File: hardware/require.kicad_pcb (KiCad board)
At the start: 6 copper layers, 68 x 26 mm, 180 parts, among them J800 Molex 47346-0001, Q110 LN235N3T5G, Q840 LMBT3904DW1T1G, SW850 SW_SKSC_4PIN, U100 RK3308, U200 SY8089AAC, U220 PAM2305CGFADJ, U230 PAM2305CGFADJ, U250 PAM2305CGFADJ, U260 NCP707_XDFN4, U300 DDR3_FBGA96, U400 EMMC_BGA_153, U500 ap6255, U830 ATECC608A-MAHDA, Y100 24MHz,12pF,10ppm, Y520 37.4MHz,12pF,10ppm

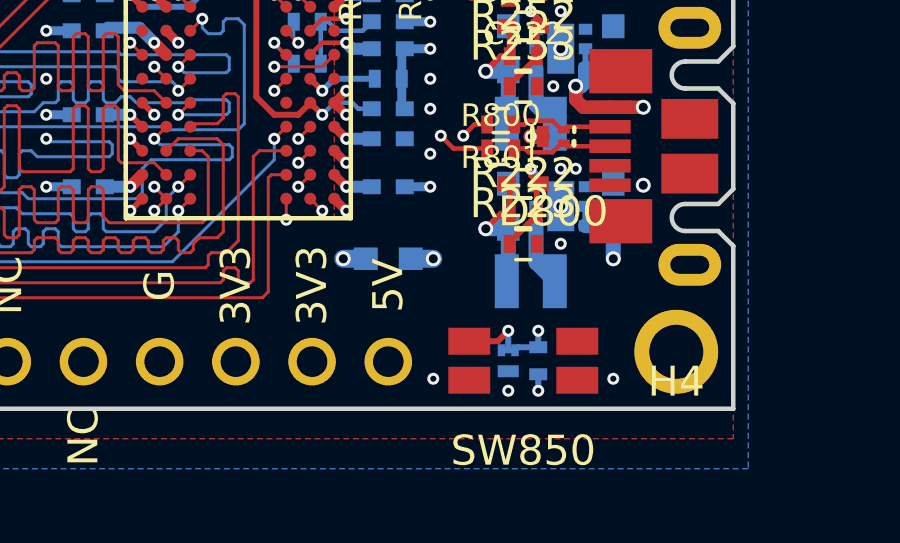
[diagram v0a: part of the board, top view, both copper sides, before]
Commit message: wip
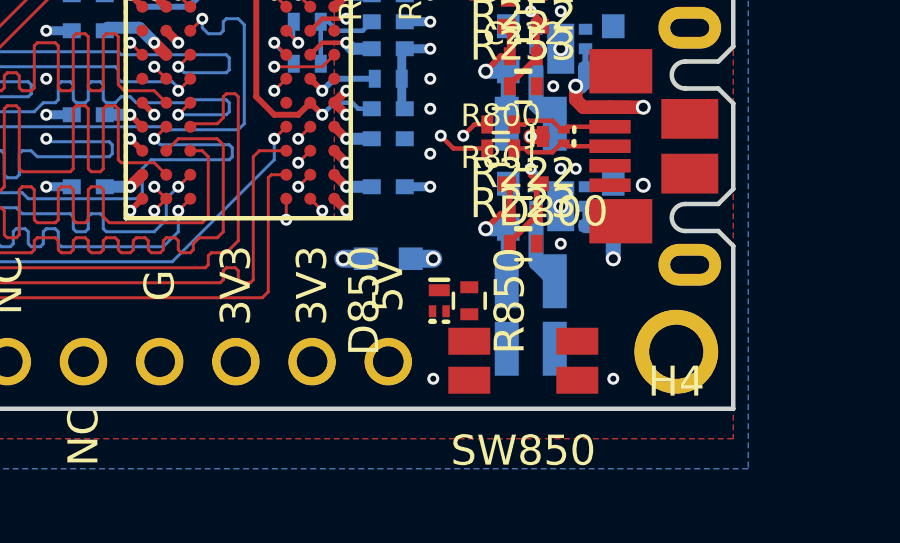
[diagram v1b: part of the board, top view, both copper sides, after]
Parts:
- added L255: 0.47u,3A, require:L_0806, B.Cu at (90.8, 76.0)
- D850, R850: moved to F.Cu
- moved D850 3.05 mm to (87.7, 74.4), turned to 90 degrees
- moved R850 3.05 mm to (88.7, 74.4), turned to 270 degrees
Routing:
- net /KEY: track 45.7 -> 31.1 mm, vias 3 -> 1
- net +3V3: track 49.2 -> 48.6 mm, vias 20 -> 19
- net GND: vias 272 -> 271

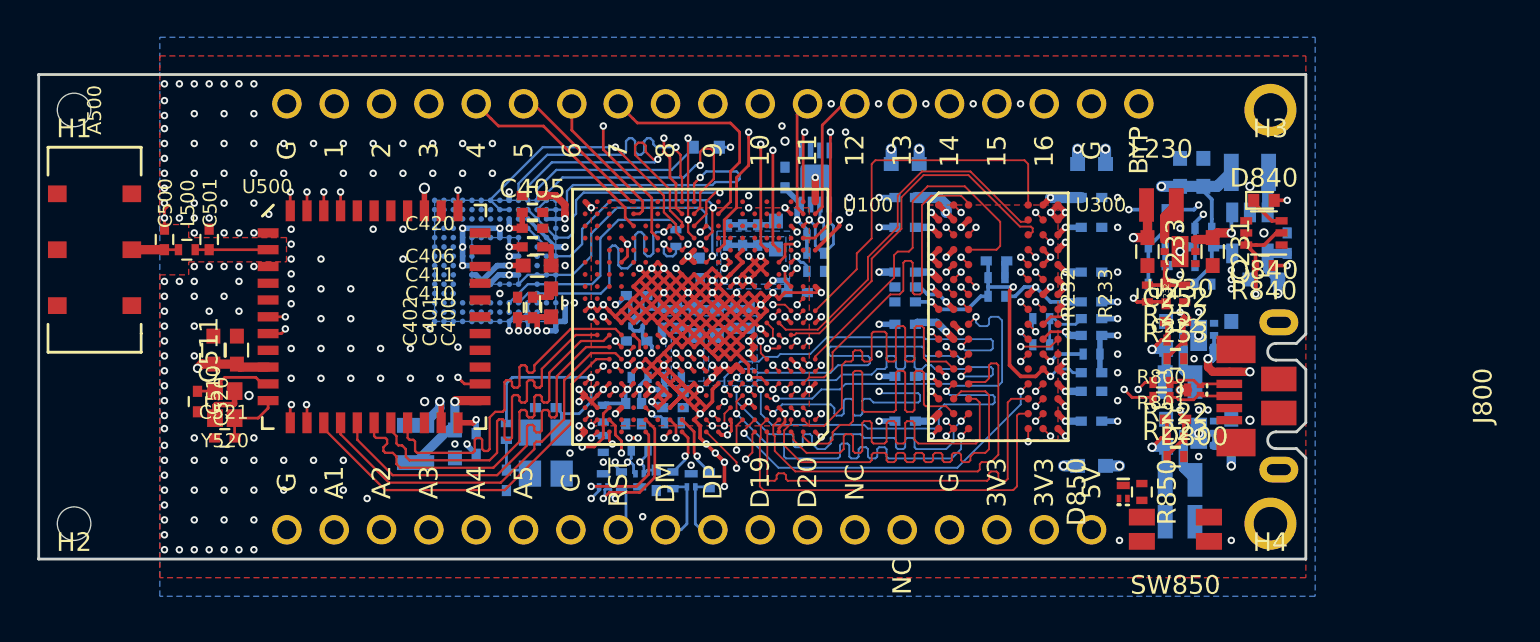
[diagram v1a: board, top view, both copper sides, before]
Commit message: wip
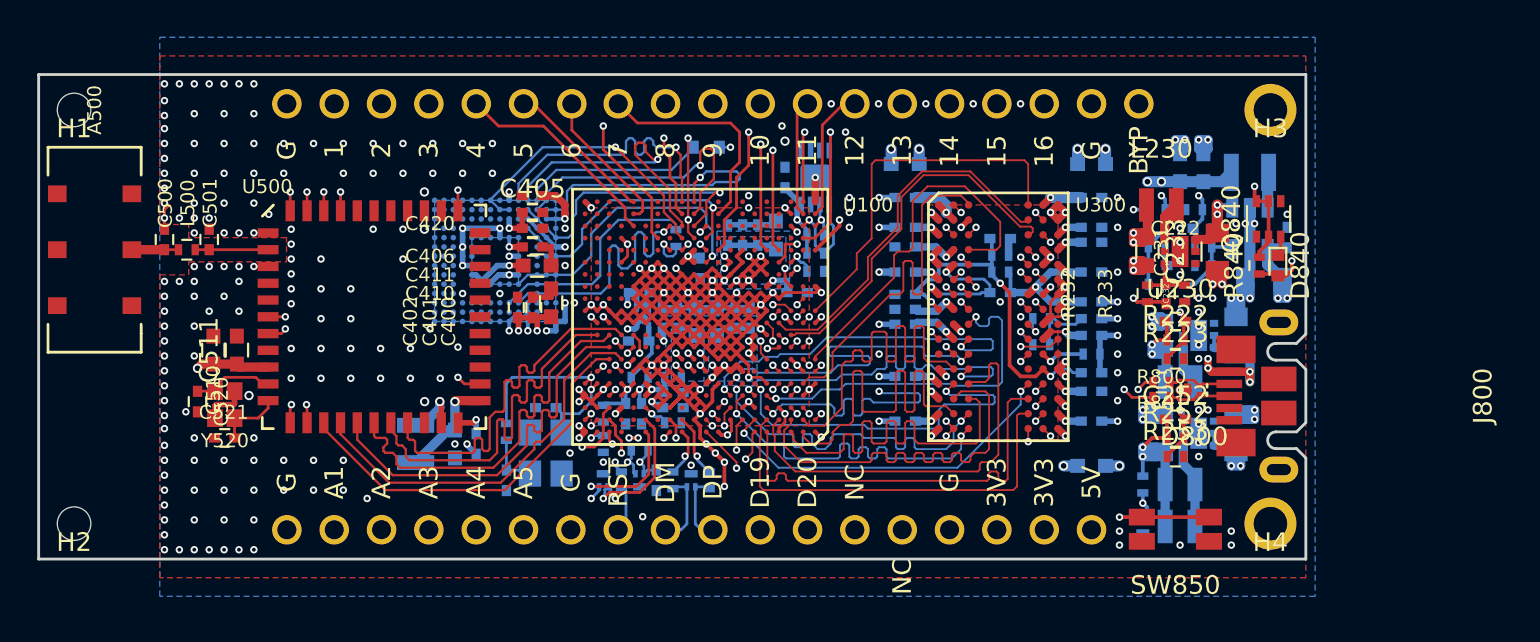
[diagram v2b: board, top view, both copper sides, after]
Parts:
- removed L255: 0.47u,3A, require:L_0806
- added C324: 0.1u, require:C_0402, B.Cu at (86.0, 61.0)
- added C325: 0.1u, require:C_0402, B.Cu at (76.0, 61.2)
- added C326: 0.1u, require:C_0402, B.Cu at (81.1, 63.7)
- added L251: 2.2u,0806, require:L_0806, B.Cu at (90.8, 76.2)
- C201, C221, C231: value 10u -> 10u,10V; footprint require:C_0603 -> require:C_0805
- C202, C222, C232, C252: value 22p -> 100p
- C210: value 0.1u -> 10n
- C223, C233: value 22u -> 10u
- C251: value 2.2u,10V -> 10u,10V; footprint require:C_0603 -> require:C_0805
- C253: value 22u -> 10u,10V; footprint require:C_0603 -> require:C_0805
- D850, R850: moved to B.Cu
- L230: value 0.47u,3A -> 2.2u
- L250: value 0.47u,3A -> 2.2u,0806
- R201: value 100R,1% -> 100R
- R210: value 10k -> 169k,1%
- R232: value 110k,1% -> 150k,1%
- R233: value 150k,1% -> 100k,1%
- R252: value 110k,1% -> 540k,1%
- R253: value 150k,1% -> 120k,1%
- moved L250 5.50 mm to (90.8, 74.0)
- moved C221 5.26 mm to (93.8, 66.0)
- moved C251 5.26 mm to (93.8, 71.2)
- moved C253 5.26 mm to (89.8, 71.2)
- moved C222 5.25 mm to (90.5, 65.2)
- moved C223 5.25 mm to (90.0, 66.0)
- moved C252 5.25 mm to (90.5, 70.5)
- moved L220 5.25 mm to (90.8, 68.5)
- moved R222 5.25 mm to (90.5, 66.2)
- moved R223 5.25 mm to (90.5, 67.2)
- moved R252 5.25 mm to (90.5, 71.5)
- moved R253 5.25 mm to (90.5, 72.5)
- moved U220 5.25 mm to (91.8, 66.0)
- moved U250 5.25 mm to (91.8, 71.2)
- moved D840 3.58 mm to (96.0, 62.2), turned to 270 degrees
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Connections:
- SW850 pad 4: Net-(SW850-Pad4) -> /KEY
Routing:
- net GND: track 246.7 -> 274.3 mm, vias 271 -> 301
- net /KEY: track 31.1 -> 48.7 mm, vias 1 -> 3
- net +5V: track 15.1 -> 21.7 mm, vias 5 -> 10
- net +3V3: track 48.6 -> 54.5 mm, vias 19 -> 18
- net +1V8: track 18.1 -> 13.3 mm, vias 3 -> 2
- net /LED: track 37.7 -> 33.2 mm
- net VCC_DDR: track 53.7 -> 56.9 mm, vias 27 -> 28
- net Net-(L250-Pad1): track 2.11 -> 4.61 mm
- net Net-(C330-Pad1): track 17.2 -> 19.1 mm
- net +1V0L: track 8.47 -> 9.82 mm, vias 7 -> 8
- net Net-(C202-Pad2): track 5.16 -> 6.16 mm
- net Net-(D840-Pad1): track 2.03 -> 1.06 mm
- net +1V0C: track 50.1 -> 49.2 mm, vias 8 -> 9

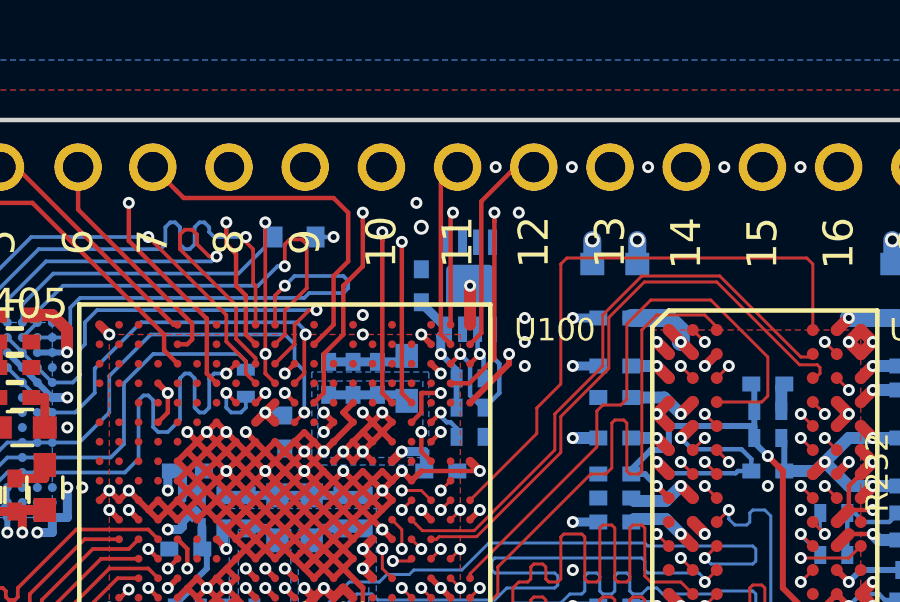
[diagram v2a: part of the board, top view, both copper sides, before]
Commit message: wip
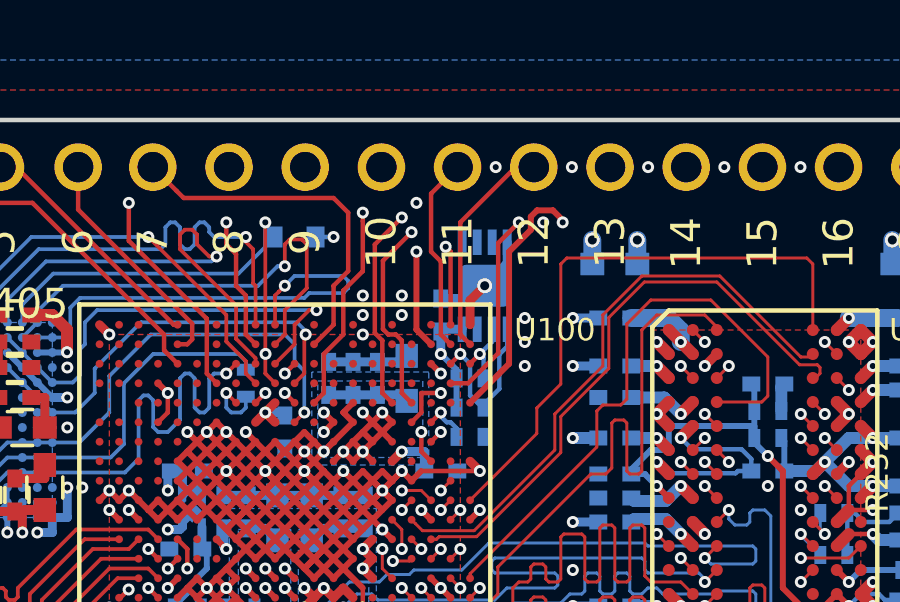
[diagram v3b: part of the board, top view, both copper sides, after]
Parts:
- moved C830 1.17 mm to (70.2, 58.5)
- moved U830 0.49 mm to (71.7, 57.5)
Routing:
- net GND: track 274.3 -> 277.9 mm, vias 301 -> 303
- net /wireless/LPO: track 31.8 -> 29.0 mm
- net /rk3308-io/D14: track 17.5 -> 14.7 mm
- net /LED: track 33.2 -> 35.2 mm
- net /KEY: track 48.7 -> 50.5 mm
- net /rk3308-io/D16: track 21.1 -> 22.1 mm
- net /rk3308-io/D13: track 11.1 -> 10.5 mm
- net +3V3: track 54.5 -> 53.8 mm
- net +1V0C: track 49.2 -> 48.6 mm
